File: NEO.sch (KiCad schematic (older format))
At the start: 13 parts, among them Q601 2N7002BKT, U601 U-BLOX-NEO-M8N, X601 ANT

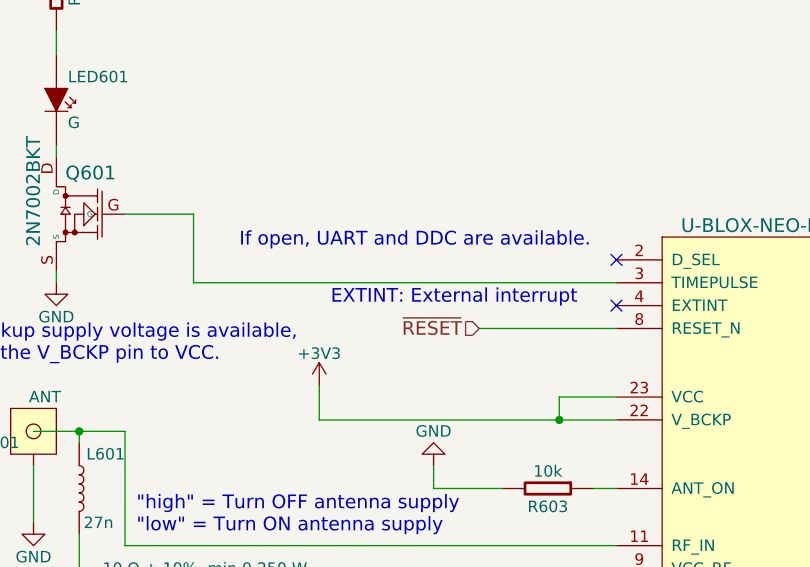
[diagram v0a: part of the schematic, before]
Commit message: sorted components
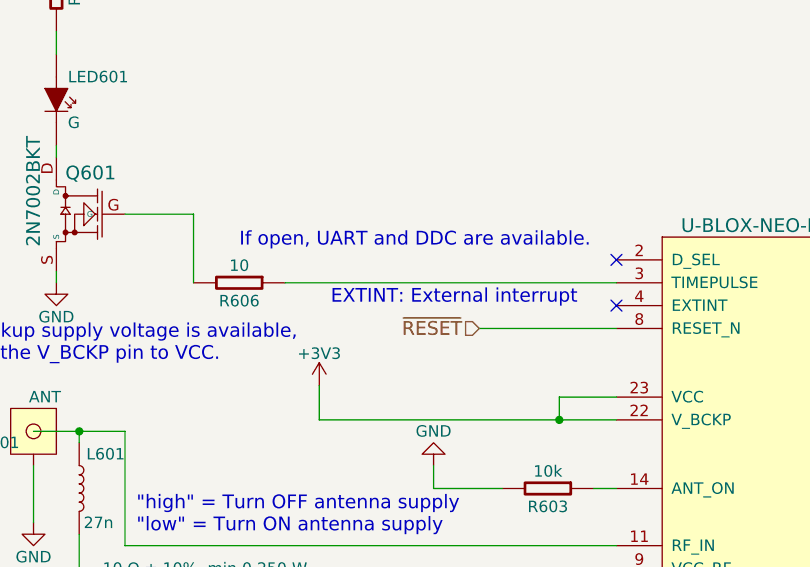
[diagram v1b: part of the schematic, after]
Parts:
- added R606: 10, Passives:R0402N, symbol R
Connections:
- net at U601.3 (TIMEPULSE): now also R606.1; no longer Q601.G
- new net: Q601.G, R606.2
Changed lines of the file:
@@
 	3950 3100 3950 2950
 $Comp
-L +3V3 #PWR0133
+L +3V3 #PWR607
 U 1 1 57190E14
 P 3950 2950
-F 0 "#PWR0133" H 3950 2800 50  0001 C CNN
+F 0 "#PWR607" H 3950 2800 50  0001 C CNN
 F 1 "+3V3" H 3950 3090 50  0000 C CNN
 F 2 "" H 3950 2950 50  0000 C CNN
@@
 $EndComp
 $Comp
-L GND #PWR0134
+L GND #PWR609
 U 1 1 57190E68
 P 7400 2900
-F 0 "#PWR0134" H 7400 2650 50  0001 C CNN
+F 0 "#PWR609" H 7400 2650 50  0001 C CNN
 F 1 "GND" H 7400 2750 50  0000 C CNN
 F 2 "" H 7400 2900 50  0000 C CNN
@@
 Connection ~ 2900 3850
 $Comp
-L GND #PWR0135
+L GND #PWR606
 U 1 1 57191865
 P 2900 4600
-F 0 "#PWR0135" H 2900 4350 50  0001 C CNN
+F 0 "#PWR606" H 2900 4350 50  0001 C CNN
 F 1 "GND" H 2900 4450 50  0000 C CNN
 F 2 "" H 2900 4600 50  0000 C CNN
@@
 $EndComp
 $Comp
-L GND #PWR0136
+L GND #PWR603
 U 1 1 57191891
 P 2700 3550
-F 0 "#PWR0136" H 2700 3300 50  0001 C CNN
+F 0 "#PWR603" H 2700 3300 50  0001 C CNN
 F 1 "GND" H 2700 3400 50  0000 C CNN
 F 2 "" H 2700 3550 50  0000 C CNN
@@
 $EndComp
 $Comp
-L GND #PWR0137
+L GND #PWR608
 U 1 1 57211964
 P 4450 3300
-F 0 "#PWR0137" H 4450 3050 50  0001 C CNN
+F 0 "#PWR608" H 4450 3050 50  0001 C CNN
 F 1 "GND" H 4450 3150 50  0000 C CNN
 F 2 "" H 4450 3300 50  0000 C CNN
@@
 $EndComp
 $Comp
-L +3V3 #PWR0138
+L +3V3 #PWR601
 U 1 1 57260BFE
 P 1200 3000
-F 0 "#PWR0138" H 1200 2850 50  0001 C CNN
+F 0 "#PWR601" H 1200 2850 50  0001 C CNN
 F 1 "+3V3" H 1200 3140 50  0000 C CNN
 F 2 "" H 1200 3000 50  0000 C CNN
@@
 $EndComp
 $Comp
-L GND #PWR0139
+L GND #PWR602
 U 1 1 57260C27
 P 1200 3800
-F 0 "#PWR0139" H 1200 3550 50  0001 C CNN
+F 0 "#PWR602" H 1200 3550 50  0001 C CNN
 F 1 "GND" H 1200 3650 50  0000 C CNN
 F 2 "" H 1200 3800 50  0000 C CNN
@@
 $EndComp
 $Comp
-L GND #PWR0140
+L GND #PWR605
 U 1 1 572B35D6
 P 2800 2500
-F 0 "#PWR0140" H 2800 2250 50  0001 C CNN
+F 0 "#PWR605" H 2800 2250 50  0001 C CNN
 F 1 "GND" H 2800 2350 50  0000 C CNN
 F 2 "" H 2800 2500 50  0000 C CNN
@@
 	2800 1400 2800 1500
 $Comp
-L +3.3V #PWR0141
+L +3.3V #PWR604
 U 1 1 572B3723
 P 2800 950
-F 0 "#PWR0141" H 2800 800 50  0001 C CNN
+F 0 "#PWR604" H 2800 800 50  0001 C CNN
 F 1 "+3.3V" H 2800 1090 50  0000 C CNN
 F 2 "" H 2800 950 50  0000 C CNN
@@
 Wire Wire Line
 	3400 2200 3400 2500
-Wire Wire Line
-	3400 2500 5250 2500
-$Comp
-L GND #PWR0142
+$Comp
+L GND #PWR610
 U 1 1 572CC1B5
 P 7450 3950
-F 0 "#PWR0142" H 7450 3700 50  0001 C CNN
+F 0 "#PWR610" H 7450 3700 50  0001 C CNN
 F 1 "GND" H 7450 3800 50  0000 C CNN
 F 2 "" H 7450 3950 50  0000 C CNN
@@
 NoConn ~ 7150 3800
 NoConn ~ 7150 3700
+$Comp
+L R R606
+U 1 1 572F007B
+P 3600 2500
+F 0 "R606" V 3680 2500 50  0000 C CNN
+F 1 "10" V 3525 2500 50  0000 C CNN
+F 2 "Passives:R0402N" V 3530 2500 30  0001 C CNN
+F 3 "" H 3600 2500 30  0000 C CNN
+	1    3600 2500
+	0    1    1    0
+$EndComp
+Wire Wire Line
+	3800 2500 5250 2500
 $EndSCHEMATC
